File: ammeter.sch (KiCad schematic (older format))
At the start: 28 parts, among them Q3 BC817, Q4 BC807, U12 LMC6482, U5 INA128

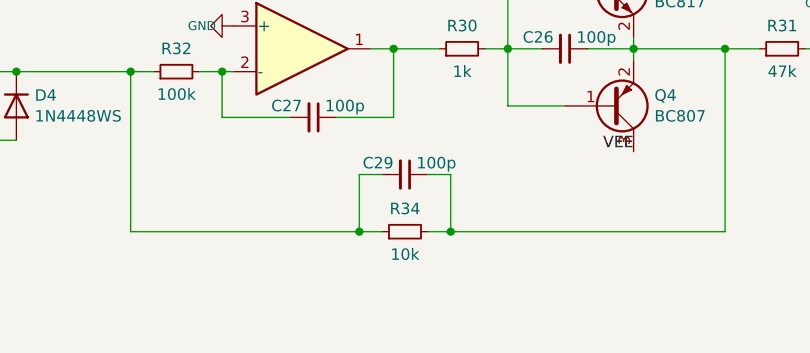
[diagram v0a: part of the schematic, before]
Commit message: - PCB progress
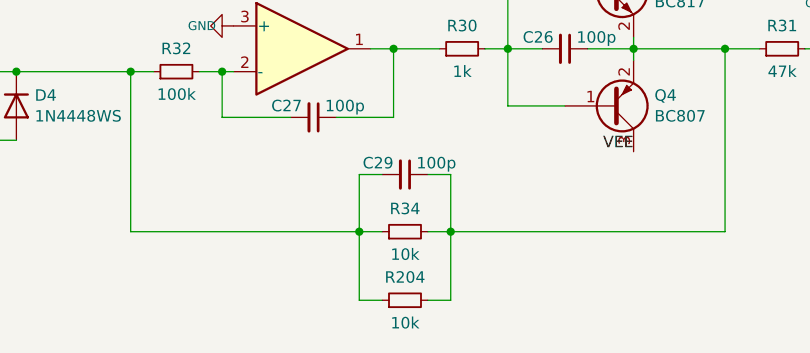
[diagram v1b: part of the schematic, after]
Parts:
- added R204: 10k, Resistor_SMD:R_1206_3216Metric, symbol Device:R_Small
- C201, C202, C25, C26, C27, C28: footprint Capacitor_SMD:C_0603_1608Metric_Pad1.05x0.95mm_HandSolder -> Capacitor_SMD:C_0603_1608Metric
- L7, L8: footprint Resistor_SMD:R_0805_2012Metric_Pad1.15x1.40mm_HandSolder -> Inductor_SMD:L_0603_1608Metric
- R14, R29, R30, R31, R33: footprint Resistor_SMD:R_0603_1608Metric_Pad1.05x0.95mm_HandSolder -> Resistor_SMD:R_0603_1608Metric
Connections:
- net at C29.2, D3.2 (A), D4.1 (K)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: now also R204.1
- net at C26.1, C29.1, Q3.2 (E)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: now also R204.2
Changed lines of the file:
@@
 F 0 "R30" V 4550 3900 50  0000 C CNN
 F 1 "1k" V 4350 3900 50  0000 C CNN
-F 2 "Resistor_SMD:R_0603_1608Metric_Pad1.05x0.95mm_HandSolder" V 4380 3900 50  0001 C CNN
+F 2 "Resistor_SMD:R_0603_1608Metric" V 4380 3900 50  0001 C CNN
 F 3 "~" H 4450 3900 50  0001 C CNN
 	1    4450 3900
@@
 F 0 "R31" V 5950 3900 50  0000 C CNN
 F 1 "47k" V 5750 3900 50  0000 C CNN
-F 2 "Resistor_SMD:R_0603_1608Metric_Pad1.05x0.95mm_HandSolder" V 5780 3900 50  0001 C CNN
+F 2 "Resistor_SMD:R_0603_1608Metric" V 5780 3900 50  0001 C CNN
 F 3 "~" H 5850 3900 50  0001 C CNN
 	1    5850 3900
@@
 F 0 "R33" V 6550 4150 50  0000 C CNN
 F 1 "47k" V 6350 4150 50  0000 C CNN
-F 2 "Resistor_SMD:R_0603_1608Metric_Pad1.05x0.95mm_HandSolder" V 6380 4150 50  0001 C CNN
+F 2 "Resistor_SMD:R_0603_1608Metric" V 6380 4150 50  0001 C CNN
 F 3 "~" H 6450 4150 50  0001 C CNN
 	1    6450 4150
@@
 F 0 "C27" V 3750 4150 50  0000 R CNN
 F 1 "100p" V 3750 4250 50  0000 L CNN
-F 2 "Capacitor_SMD:C_0603_1608Metric_Pad1.05x0.95mm_HandSolder" H 3800 4200 50  0001 C CNN
+F 2 "Capacitor_SMD:C_0603_1608Metric" H 3800 4200 50  0001 C CNN
 F 3 "~" H 3800 4200 50  0001 C CNN
 	1    3800 4200
@@
 F 0 "C26" V 4850 3850 50  0000 R CNN
 F 1 "100p" V 4850 3950 50  0000 L CNN
-F 2 "Capacitor_SMD:C_0603_1608Metric_Pad1.05x0.95mm_HandSolder" H 4900 3900 50  0001 C CNN
+F 2 "Capacitor_SMD:C_0603_1608Metric" H 4900 3900 50  0001 C CNN
 F 3 "~" H 4900 3900 50  0001 C CNN
 	1    4900 3900
@@
 F 0 "R29" V 7300 3800 50  0000 C CNN
 F 1 "1k" V 7100 3800 50  0000 C CNN
-F 2 "Resistor_SMD:R_0603_1608Metric_Pad1.05x0.95mm_HandSolder" V 7130 3800 50  0001 C CNN
+F 2 "Resistor_SMD:R_0603_1608Metric" V 7130 3800 50  0001 C CNN
 F 3 "~" H 7200 3800 50  0001 C CNN
 	1    7200 3800
@@
 F 0 "C25" H 8350 3900 50  0000 L CNN
 F 1 "100n" H 8350 3800 50  0000 L CNN
-F 2 "Capacitor_SMD:C_0603_1608Metric_Pad1.05x0.95mm_HandSolder" H 8250 3850 50  0001 C CNN
+F 2 "Capacitor_SMD:C_0603_1608Metric" H 8250 3850 50  0001 C CNN
 F 3 "~" H 8250 3850 50  0001 C CNN
 	1    8250 3850
@@
 F 0 "L7" V 8855 3750 50  0000 C CNN
 F 1 "BLM18RK102" V 8764 3750 50  0000 C CNN
-F 2 "Resistor_SMD:R_0805_2012Metric_Pad1.15x1.40mm_HandSolder" H 8650 3750 50  0001 C CNN
+F 2 "Inductor_SMD:L_0603_1608Metric" H 8650 3750 50  0001 C CNN
 F 3 "~" H 8650 3750 50  0001 C CNN
 	1    8650 3750
@@
 F 0 "C28" H 8350 4300 50  0000 L CNN
 F 1 "100n" H 8350 4200 50  0000 L CNN
-F 2 "Capacitor_SMD:C_0603_1608Metric_Pad1.05x0.95mm_HandSolder" H 8250 4250 50  0001 C CNN
+F 2 "Capacitor_SMD:C_0603_1608Metric" H 8250 4250 50  0001 C CNN
 F 3 "~" H 8250 4250 50  0001 C CNN
 	1    8250 4250
@@
 F 0 "L8" V 8855 4350 50  0000 C CNN
 F 1 "BLM18RK102" V 8764 4350 50  0000 C CNN
-F 2 "Resistor_SMD:R_0805_2012Metric_Pad1.15x1.40mm_HandSolder" H 8650 4350 50  0001 C CNN
+F 2 "Inductor_SMD:L_0603_1608Metric" H 8650 4350 50  0001 C CNN
 F 3 "~" H 8650 4350 50  0001 C CNN
 	1    8650 4350
@@
 F 0 "C201" H 4750 1600 50  0000 L CNN
 F 1 "100n" H 4750 1500 50  0000 L CNN
-F 2 "Capacitor_SMD:C_0603_1608Metric_Pad1.05x0.95mm_HandSolder" H 4650 1550 50  0001 C CNN
+F 2 "Capacitor_SMD:C_0603_1608Metric" H 4650 1550 50  0001 C CNN
 F 3 "~" H 4650 1550 50  0001 C CNN
 	1    4650 1550
@@
 F 0 "C202" H 4500 2550 50  0000 L CNN
 F 1 "100n" H 4500 2450 50  0000 L CNN
-F 2 "Capacitor_SMD:C_0603_1608Metric_Pad1.05x0.95mm_HandSolder" H 4400 2500 50  0001 C CNN
+F 2 "Capacitor_SMD:C_0603_1608Metric" H 4400 2500 50  0001 C CNN
 F 3 "~" H 4400 2500 50  0001 C CNN
 	1    4400 2500
@@
 F 0 "R14" V 2800 1800 50  0000 C CNN
 F 1 "100k" V 2600 1800 50  0000 C CNN
-F 2 "Resistor_SMD:R_0603_1608Metric_Pad1.05x0.95mm_HandSolder" V 2630 1800 50  0001 C CNN
+F 2 "Resistor_SMD:R_0603_1608Metric" V 2630 1800 50  0001 C CNN
 F 3 "~" H 2700 1800 50  0001 C CNN
 	1    2700 1800
@@
 Wire Wire Line
 	6800 3300 6800 3800
+$Comp
+L Device:R_Small R?
+U 1 1 5FA9EA22
+P 4200 5000
+AR Path="/5F40DCB9/5FA9EA22" Ref="R?"  Part="1"
+AR Path="/5F618AB9/5FA9EA22" Ref="R204"  Part="1"
+F 0 "R204" V 4300 5000 50  0000 C CNN
+F 1 "10k" V 4100 5000 50  0000 C CNN
+F 2 "Resistor_SMD:R_1206_3216Metric" V 4130 5000 50  0001 C CNN
+F 3 "~" H 4200 5000 50  0001 C CNN
+	1    4200 5000
+	0    -1   -1   0
+$EndComp
+Wire Wire Line
+	4100 5000 4000 5000
+Wire Wire Line
+	4000 4700 4000 5000
+Wire Wire Line
+	4400 5000 4400 4700
+Wire Wire Line
+	4300 5000 4400 5000
 $EndSCHEMATC
